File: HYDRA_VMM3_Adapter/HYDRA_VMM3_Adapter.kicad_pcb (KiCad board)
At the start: 10 copper layers, 121.5 x 31.5 mm, 7 parts, among them J1 ME1014010101011, J2 ME1014010101011, J3 ME1014010101011, J4 ME1014010101011, J5 ME1014010101011, J6 ME1014010101011

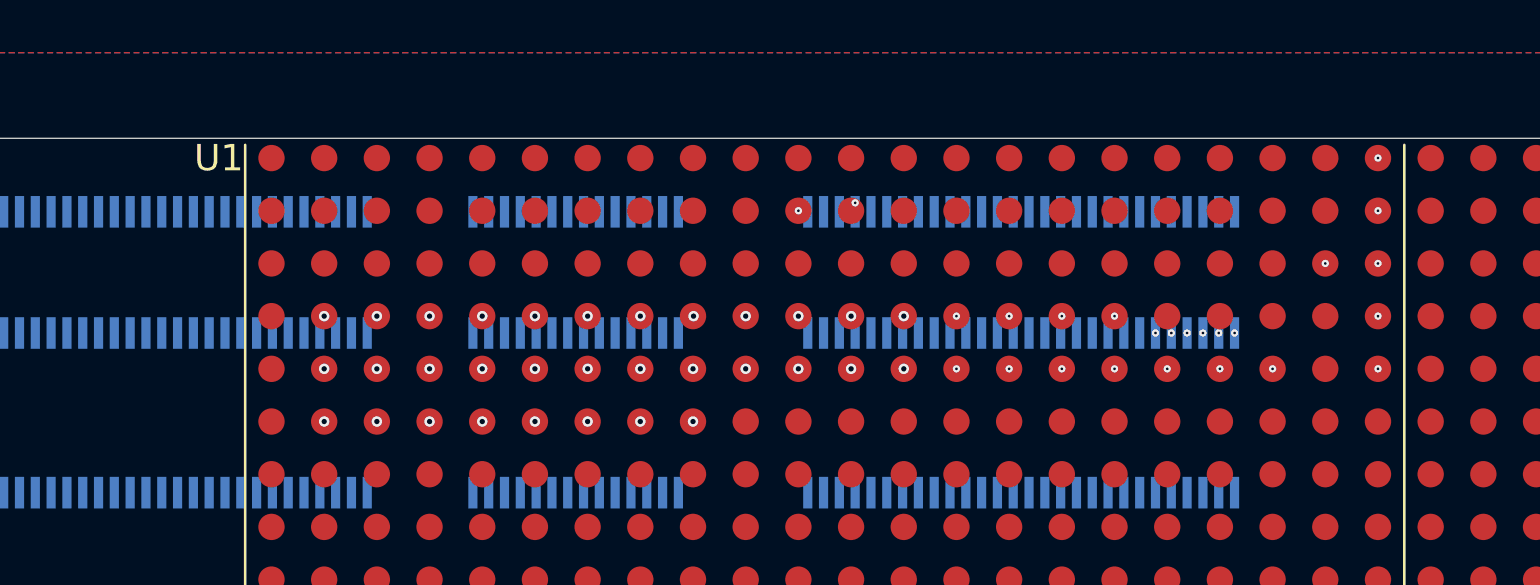
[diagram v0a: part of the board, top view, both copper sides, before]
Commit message: .
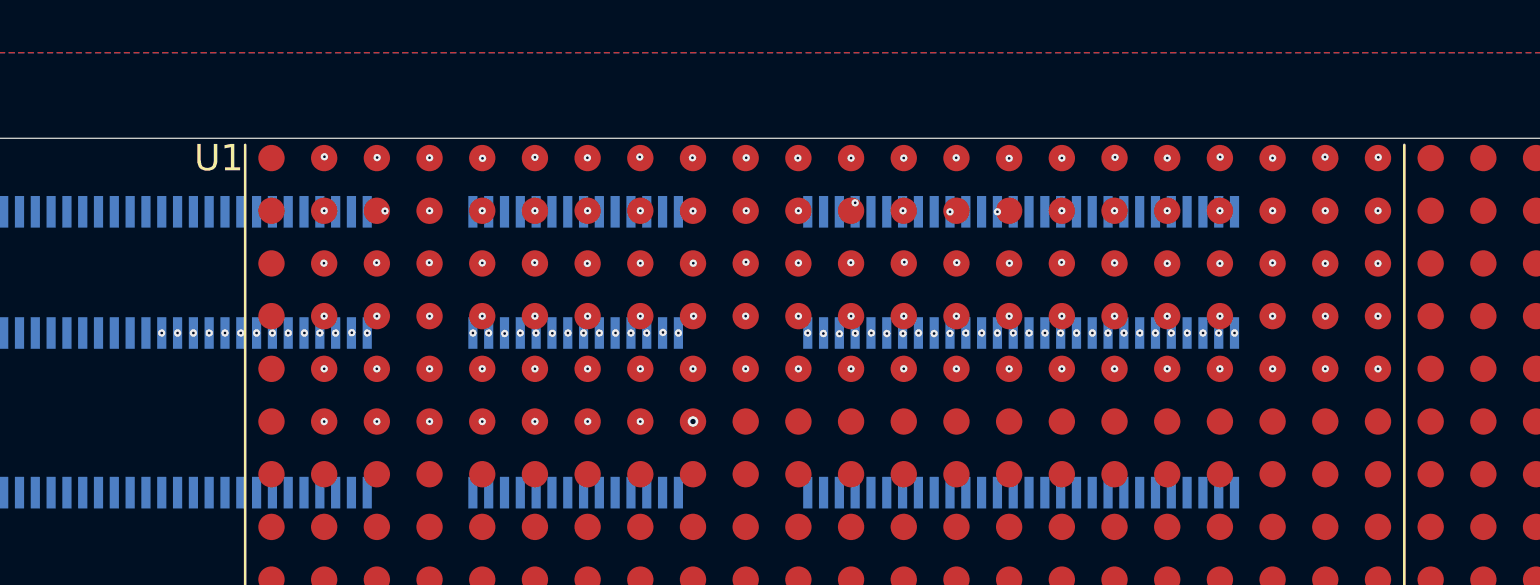
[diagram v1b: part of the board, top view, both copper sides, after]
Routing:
- net Col_22-Row_1: track 11.9 -> 0.04 mm
- net Col_22-Row_2: track 9.14 -> 0.00 mm
- net Col_22-Row_5: track 8.43 -> 0.02 mm
- net Col_22-Row_4: track 8.00 -> 0.00 mm
- net Col_21-Row_3: track 7.65 -> 0.00 mm
- net Col_22-Row_3: track 6.80 -> 0.00 mm
- net Col_3-Row_2: track 0.00 -> 0.31 mm, vias 0 -> 1
- net Col_14-Row_2: track 0.02 -> 0.28 mm, vias 0 -> 1
- net Col_13-Row_3: track 0.00 -> 0.06 mm, vias 0 -> 1
- net Col_2-Row_1: track 0.00 -> 0.05 mm, vias 0 -> 1
- net Col_10-Row_3: track 0.00 -> 0.05 mm, vias 0 -> 1
- net Col_8-Row_1: track 0.00 -> 0.05 mm, vias 0 -> 1
- net Col_19-Row_3: track 0.00 -> 0.04 mm, vias 0 -> 1
- net Col_21-Row_1: track 0.00 -> 0.04 mm, vias 0 -> 2
- net Col_16-Row_3: track 0.00 -> 0.04 mm, vias 0 -> 1
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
